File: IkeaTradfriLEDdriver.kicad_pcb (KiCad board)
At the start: 2 copper layers, 89.5 x 39.4 mm, 19 parts, among them J1 zdroj, J2 IKEA Zigbit module, J3 led strip, Q1 BUZ11, Q2 BC547, U1 LM741, U2 LM1117-3.3

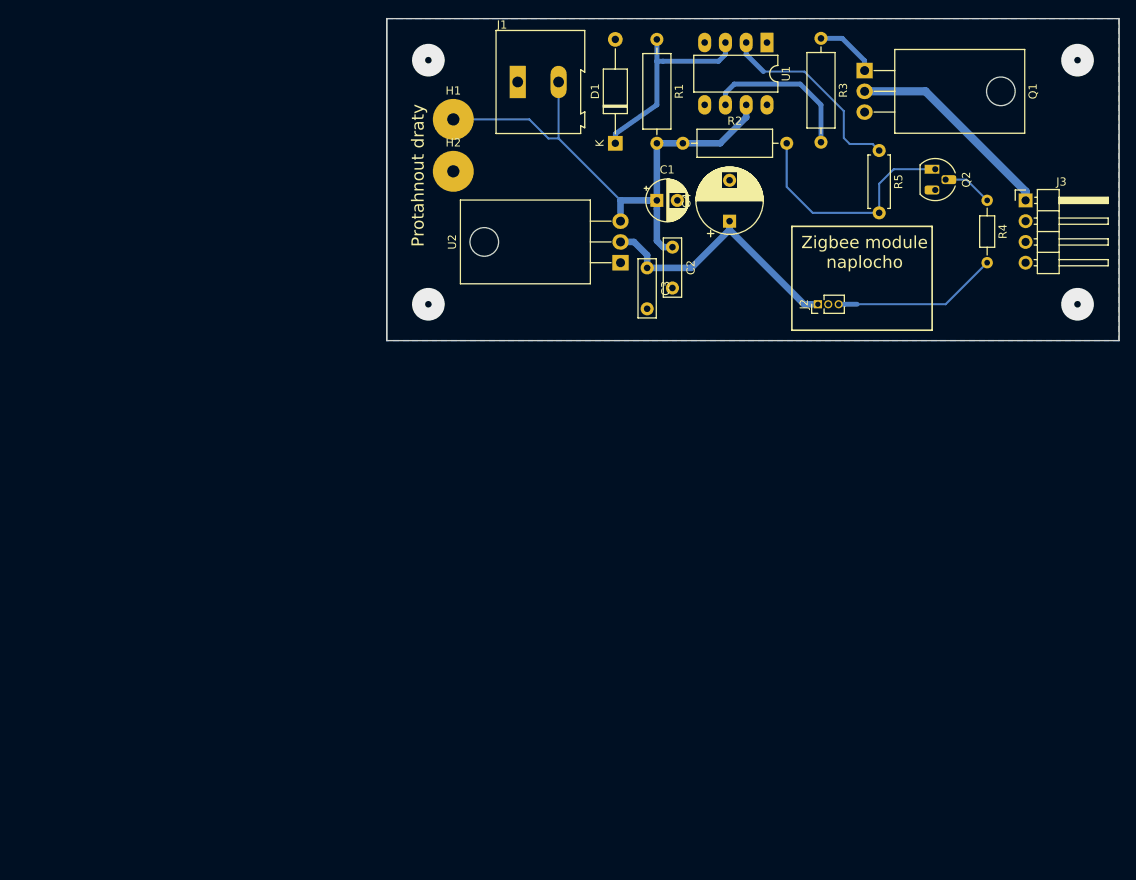
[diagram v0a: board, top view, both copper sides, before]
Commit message: Nova deska + gerber soubory
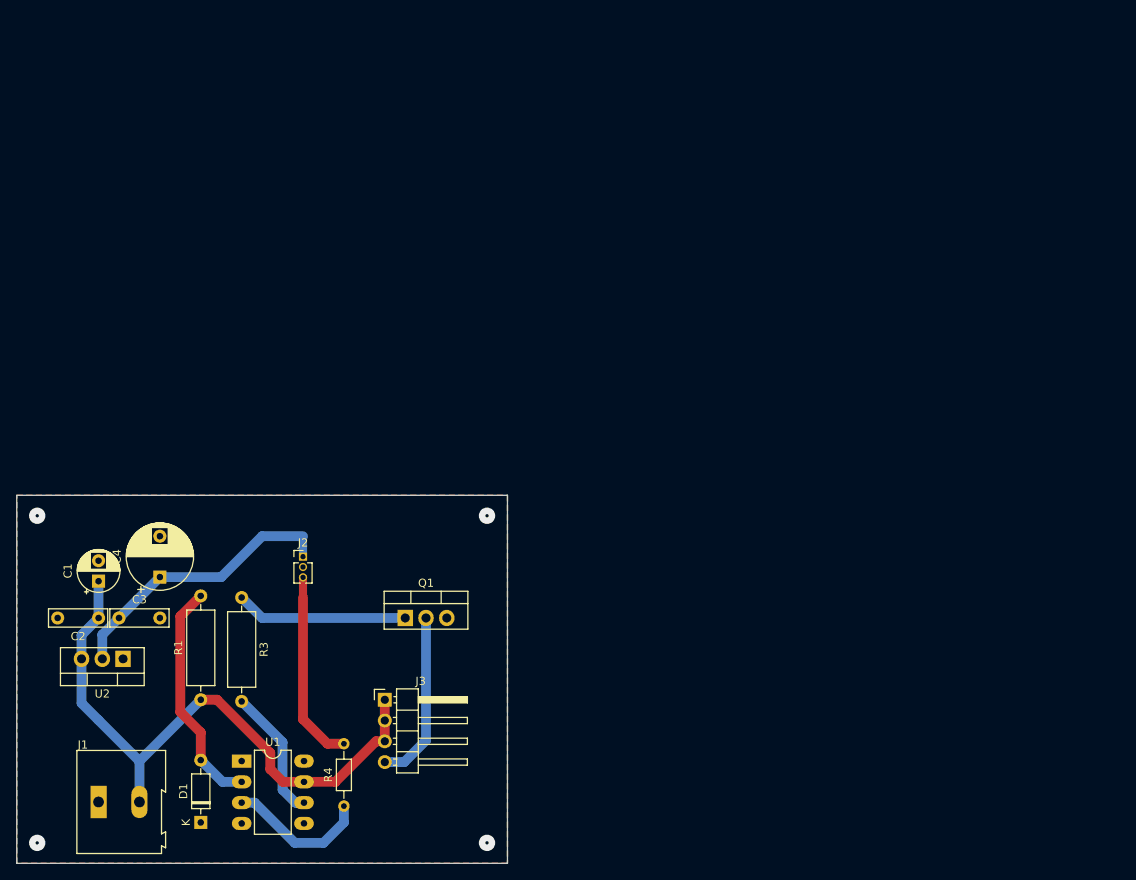
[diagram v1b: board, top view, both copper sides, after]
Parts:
- removed H1: +, MountingHole:MountingHole_2.5mm_Pad
- removed H2: -, MountingHole:MountingHole_2.5mm_Pad
- removed Q2: BC547, Package_TO_SOT_THT:TO-92L_HandSolder
- removed R2: 10k, Resistor_THT:R_Axial_DIN0309_L9.0mm_D3.2mm_P12.70mm_Horizontal
- removed R5: 10k, Resistor_THT:R_Axial_DIN0207_L6.3mm_D2.5mm_P7.62mm_Horizontal
- D1: value D_Zener -> 1N4148; footprint Diode_THT:D_A-405_P12.70mm_Horizontal -> Diode_THT:D_DO-35_SOD27_P7.62mm_Horizontal
- Q1, U2: footprint Package_TO_SOT_THT:TO-220-3_Horizontal_TabDown -> Package_TO_SOT_THT:TO-220-3_Vertical
- R3: value 120 -> 220
- moved U1 108.8 mm to (77.5, 160.0), turned to 0 degrees
- moved R4 108.0 mm to (90.0, 165.5), turned to 90 degrees
- moved J1 101.9 mm to (60.0, 165.0)
- moved J3 99.3 mm to (95.0, 152.5)
- moved R3 98.5 mm to (77.5, 140.0)
- moved R1 98.1 mm to (72.5, 152.5), turned to 90 degrees
- moved D1 97.3 mm to (72.5, 167.5)
- moved Q1 87.4 mm to (97.5, 142.5), turned to 0 degrees
- moved C2 83.6 mm to (60.0, 142.5), turned to 180 degrees
- moved C1 82.6 mm to (60.0, 138.0), turned to 90 degrees
- moved C4 82.1 mm to (67.5, 137.5)
- moved U2 77.8 mm to (63.0, 147.5), turned to 180 degrees
- moved C3 77.5 mm to (62.5, 142.5), turned to 0 degrees
- moved J2 70.1 mm to (85.0, 135.0), turned to 0 degrees
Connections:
- D1 pad 1: Net-(D1-Pad1) -> GND
- D1 pad 2: GND -> Net-(D1-Pad2)
- J3 pad 1: Net-(J3-Pad1) -> +12V
- J3 pad 2: Net-(J3-Pad1) -> +12V
- J3 pad 3: Net-(J3-Pad1) -> +12V
- J3 pad 4: GND -> Net-(J3-Pad4)
- Q1 pad 2: Net-(J3-Pad1) -> Net-(J3-Pad4)
- R1 pad 1: Net-(D1-Pad1) -> +12V
- R1 pad 2: +12V -> Net-(D1-Pad2)
- R4 pad 1: Net-(Q2-Pad2) -> Net-(R4-Pad1)
- U1 pad 2: Net-(R5-Pad1) -> Net-(D1-Pad2)
- U1 pad 3: Net-(D1-Pad1) -> Net-(R4-Pad1)
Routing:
- net Net-(Q2-Pad1): track 29.1 -> 0.00 mm
- net Net-(D1-Pad2): track 0.00 -> 28.3 mm
- net Net-(J3-Pad1): track 25.9 -> 0.00 mm
- net Net-(D1-Pad1): track 25.5 -> 0.00 mm
- net Net-(R5-Pad1): track 24.5 -> 0.00 mm
- net Net-(J3-Pad4): track 0.00 -> 21.1 mm
- net Net-(R4-Pad1): track 0.00 -> 17.6 mm
- net +12V: track 66.4 -> 81.7 mm
- net Net-(Q1-Pad1): track 7.72 -> 21.1 mm
- net Net-(Q2-Pad2): track 6.13 -> 0.00 mm
- net pwm: track 20.3 -> 26.0 mm
- net Net-(R3-Pad2): track 19.2 -> 16.1 mm
- net +3V3: track 33.1 -> 35.0 mm
- added copper zone on F.Cu, net GND
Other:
- board size 89.5 x 39.4 mm -> 60 x 45 mm
- net class Default: trace_width 0.25 -> 1.2
- board text removed: "Protahnout draty"
- board text removed: "Zigbee module naplocho"
